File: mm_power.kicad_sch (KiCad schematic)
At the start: 1 part, among them J5 Conn_01x02

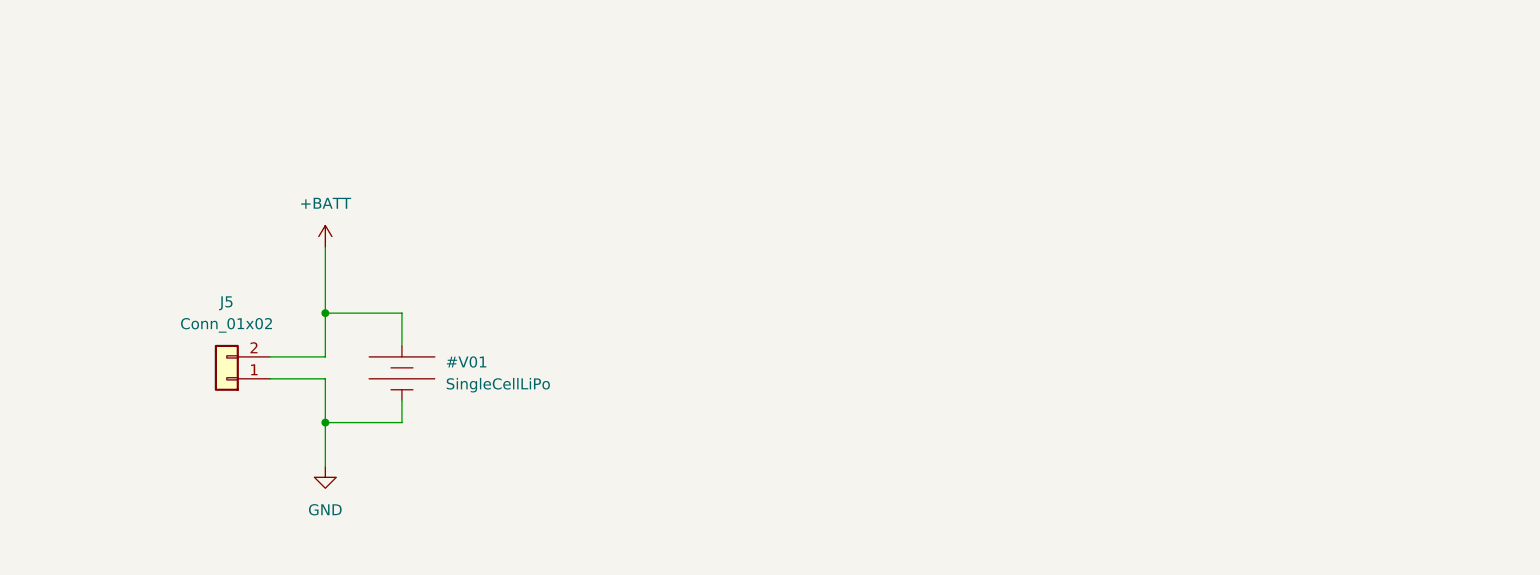
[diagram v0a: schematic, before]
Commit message: fin tp2
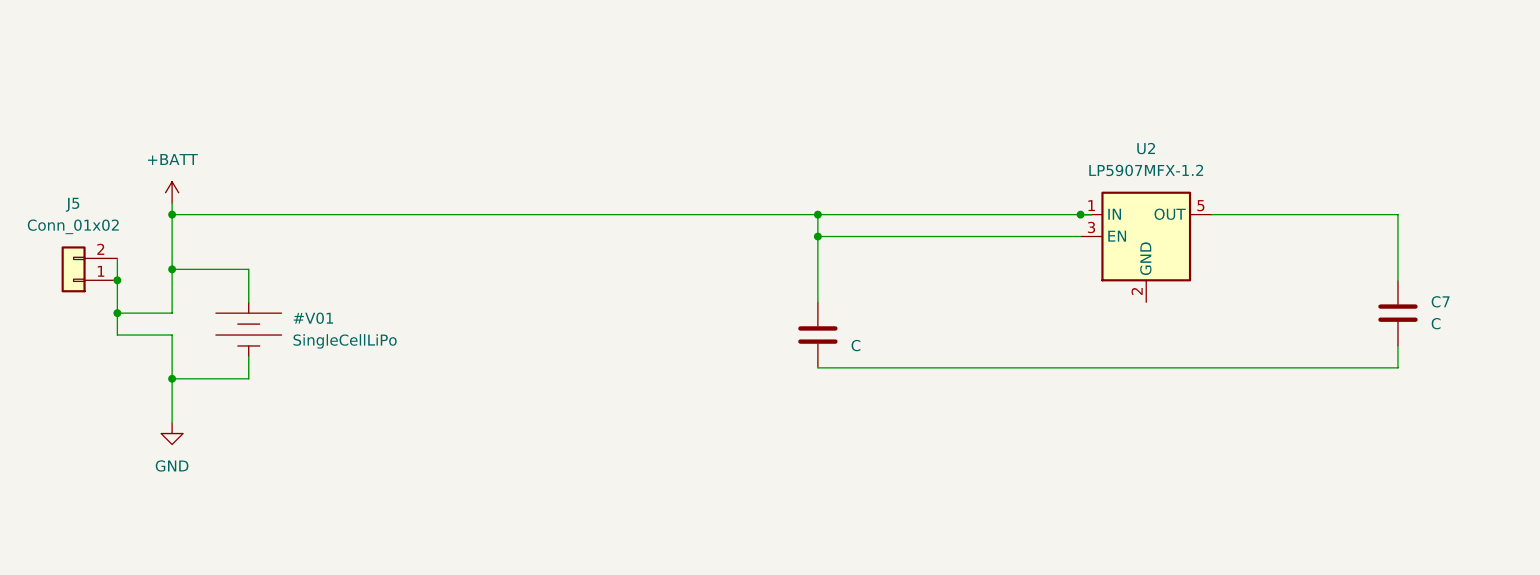
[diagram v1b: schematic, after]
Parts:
- added C7, C8: C, symbol Device:C
- added U2: LP5907MFX-1.2, Package_TO_SOT_SMD:SOT-23-5, symbol Regulator_Linear:LP5907MFX-1.2
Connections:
- net GND is gone; now on net +BATT: J5.1 (Pin_1)
- net +BATT: now also C8.1, U2.1 (IN), U2.3 (EN)
- new net: C7.2, C8.2
- new net: C7.1, U2.5 (OUT)
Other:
- moved on the sheet: J5

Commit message: tp3
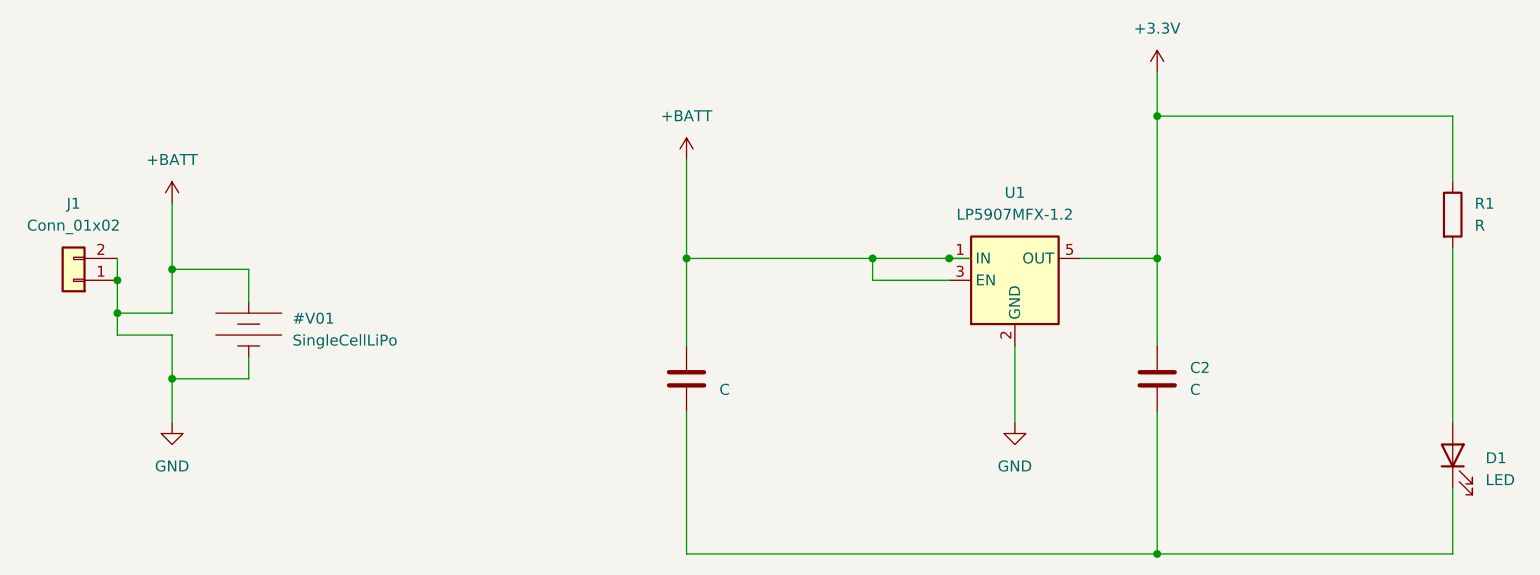
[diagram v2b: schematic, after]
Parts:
- added D1: LED, LED_SMD:LED_0603_1608Metric, symbol Device:LED
- added R1: R, Resistor_SMD:R_0603_1608Metric, symbol Device:R
- C1: renamed from C8; footprint (none) -> Capacitor_SMD:C_0603_1608Metric
- C2: renamed from C7; footprint (none) -> Capacitor_SMD:C_0603_1608Metric
- renumbered J5 to J1, U2 to U1
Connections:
- net +BATT: now also U1.2 (GND)
- net at C1.2, C2.2: now also D1.1 (K)
- net +3.3V: now reaches C2.1, U1.5 (OUT)
- net +3.3V: now also R1.1
- new net: D1.2 (A), R1.2
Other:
- moved on the sheet: C2, U1
